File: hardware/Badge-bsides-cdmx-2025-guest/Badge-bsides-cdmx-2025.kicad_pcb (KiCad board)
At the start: 2 copper layers, 50 x 110 mm, 30 parts, among them J1 SWDIO, J3 ADDON, J4 Conn_01x04_Pin, J5 I2C, J6 Conn_01x04_Pin, P6 USB_C_Plug_USB2.0, Q3 DMG3415U-7, SW11 ON, SW2 RESET, U1 PY32F030F28U6TR, U6 AP2112K-3.3

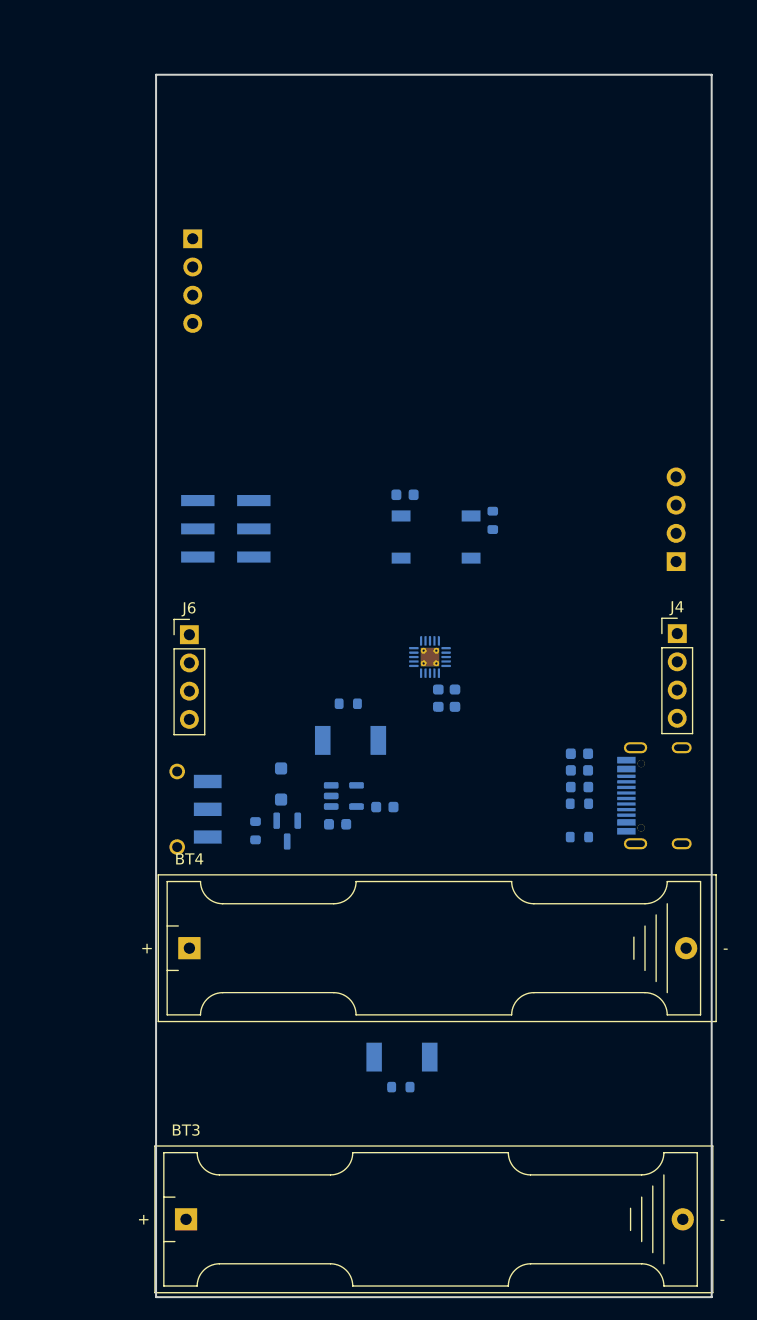
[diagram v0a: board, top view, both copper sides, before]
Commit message: feat(Hw):started_routing
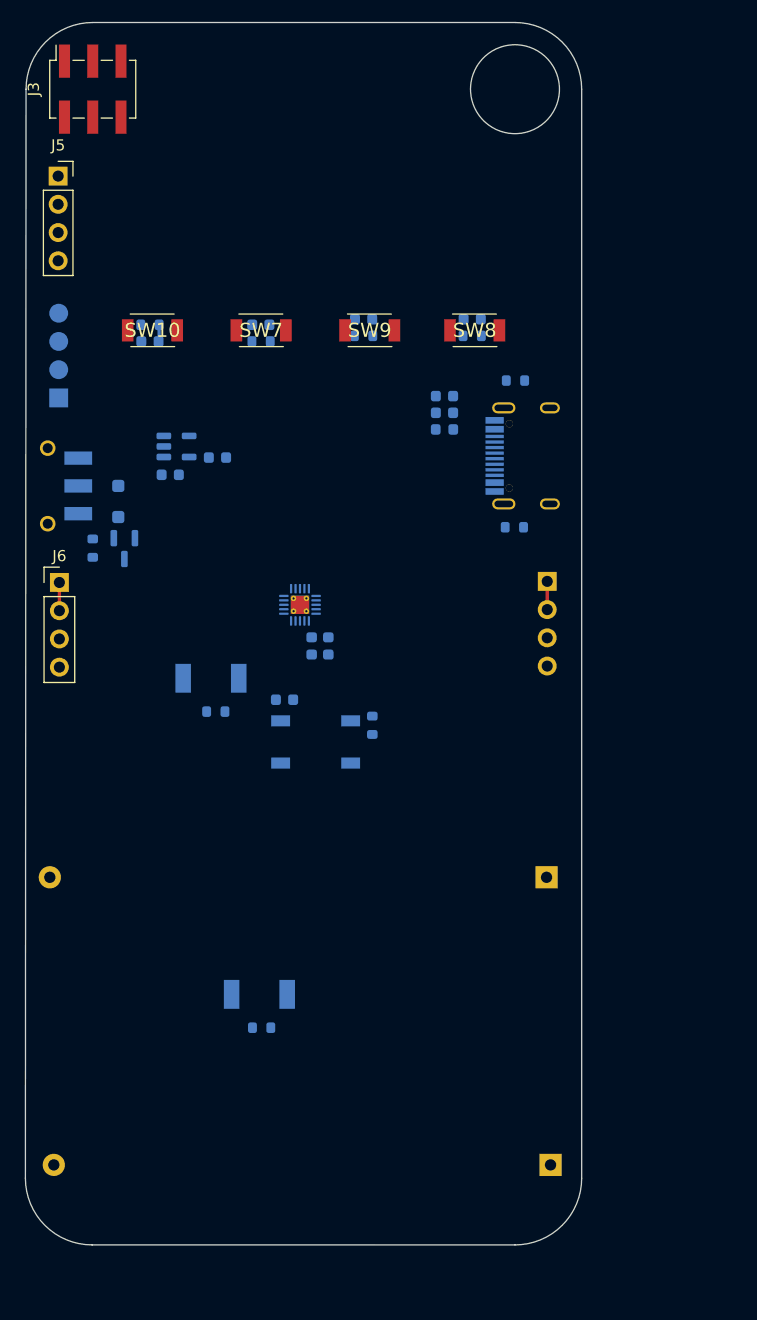
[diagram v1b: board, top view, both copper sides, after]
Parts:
- added C67: 10uF, Capacitor_SMD:C_0603_1608Metric, B.Cu at (153.4, 61.0)
- added C68: 10uF, Capacitor_SMD:C_0603_1608Metric, B.Cu at (143.7, 61.0)
- added C69: 10uF, Capacitor_SMD:C_0603_1608Metric, B.Cu at (134.4, 61.5)
- added C70: 10uF, Capacitor_SMD:C_0603_1608Metric, B.Cu at (124.5, 63.0)
- added R5: 10k, Resistor_SMD:R_0603_1608Metric, B.Cu at (153.4, 62.5)
- added R6: 10k, Resistor_SMD:R_0603_1608Metric, B.Cu at (143.7, 62.5)
- added R7: 10k, Resistor_SMD:R_0603_1608Metric, B.Cu at (134.4, 63.0)
- added R8: 10k, Resistor_SMD:R_0603_1608Metric, B.Cu at (124.5, 61.5)
- added SW10: SW_Push, Footprints:TS1088R02026, F.Cu at (124.7, 62.0)
- added SW7: SW_Push, Footprints:TS1088R02026, F.Cu at (134.4, 62.0)
- added SW8: SW_Push, Footprints:TS1088R02026, F.Cu at (153.7, 62.0)
- added SW9: SW_Push, Footprints:TS1088R02026, F.Cu at (144.2, 62.0)
- BT3, BT4, J4: moved to B.Cu
- J3, J5: moved to F.Cu
- moved J1 57.5 mm to (116.2, 68.1)
- moved BT3 44.7 mm to (160.1, 111.2), turned to 180 degrees
- moved J3 41.3 mm to (119.3, 40.3), turned to 90 degrees
- moved R41 38.5 mm to (157.3, 66.5)
- moved D10 38.2 mm to (129.9, 93.3)
- moved BT4 37.9 mm to (160.5, 137.1), turned to 180 degrees
- moved R11 37.7 mm to (130.4, 96.3), turned to 180 degrees
- moved C33 35.8 mm to (151.0, 67.9)
- moved C10 34.9 mm to (126.3, 75.0)
- moved C26 34.9 mm to (130.5, 73.5)
- moved U6 34.9 mm to (126.8, 72.5)
- moved F3 34.4 mm to (151.0, 70.9)
- moved C27 33.0 mm to (151.0, 69.4)
- moved P6 32.8 mm to (156.3, 73.3)
- moved SW11 31.3 mm to (117.0, 76.0)
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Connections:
- BT3 pad 2: +3.3V -> +BATT
- J3 pad 5: /GPIO1 -> /GPIO2
- J3 pad 6: /GPIO2 -> /GPIO1
- U1 pad 1: unconnected-(U1-PA5-Pad1) -> /BTTN2
- U1 pad 10: unconnected-(U1-PB6-Pad10) -> /LED1
- U1 pad 16: /GPIO2 -> /BTTN4
- U1 pad 17: /GPIO1 -> /BTTN3
- U1 pad 2: /LED1 -> /BTTN1
- U1 pad 20: unconnected-(U1-PA4-Pad20) -> /LED2
- U1 pad 3: /LED2 -> /GPIO1
- U1 pad 5: unconnected-(U1-PA12-Pad5) -> /GPIO2
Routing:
- net /TX: track 0.00 -> 2.54 mm
- net /RX: track 0.00 -> 2.54 mm
- net /BTTN4: track 0.00 -> 1.52 mm
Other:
- board size 50 x 110 mm -> 50.1 x 110 mm
